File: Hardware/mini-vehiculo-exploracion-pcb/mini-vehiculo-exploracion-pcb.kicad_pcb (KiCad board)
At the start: 2 copper layers, 82 parts, among them IC3 MAX8891EXK33_V+T, J1 Cámara, J2 USB_C_Receptacle_USB2.0_16P, J4 MOTORES, J8 SERVO, Q1 SI1467DH-T1-BE3, U2 ESP32-S3-WROOM-1, U3 LM358, U4 TPS561208DDCR, Y1 830003000

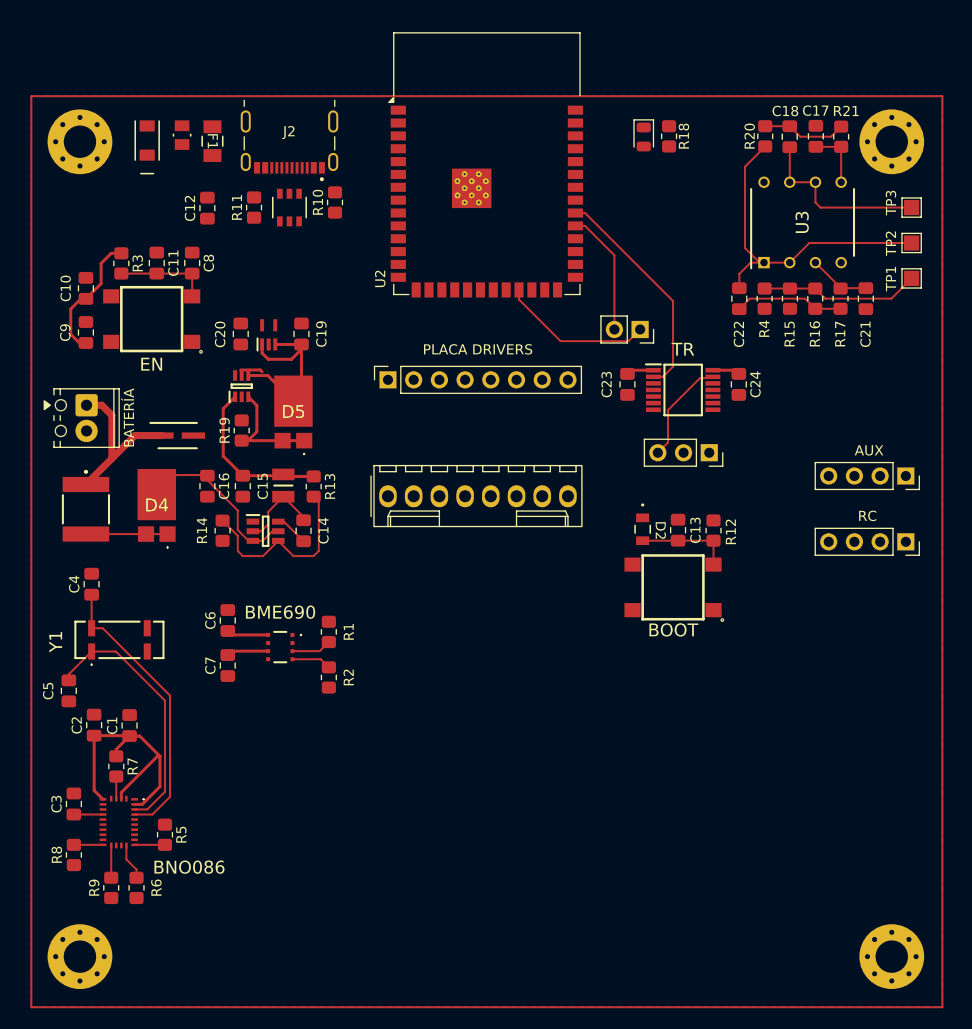
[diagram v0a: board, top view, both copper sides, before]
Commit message: update pcb3
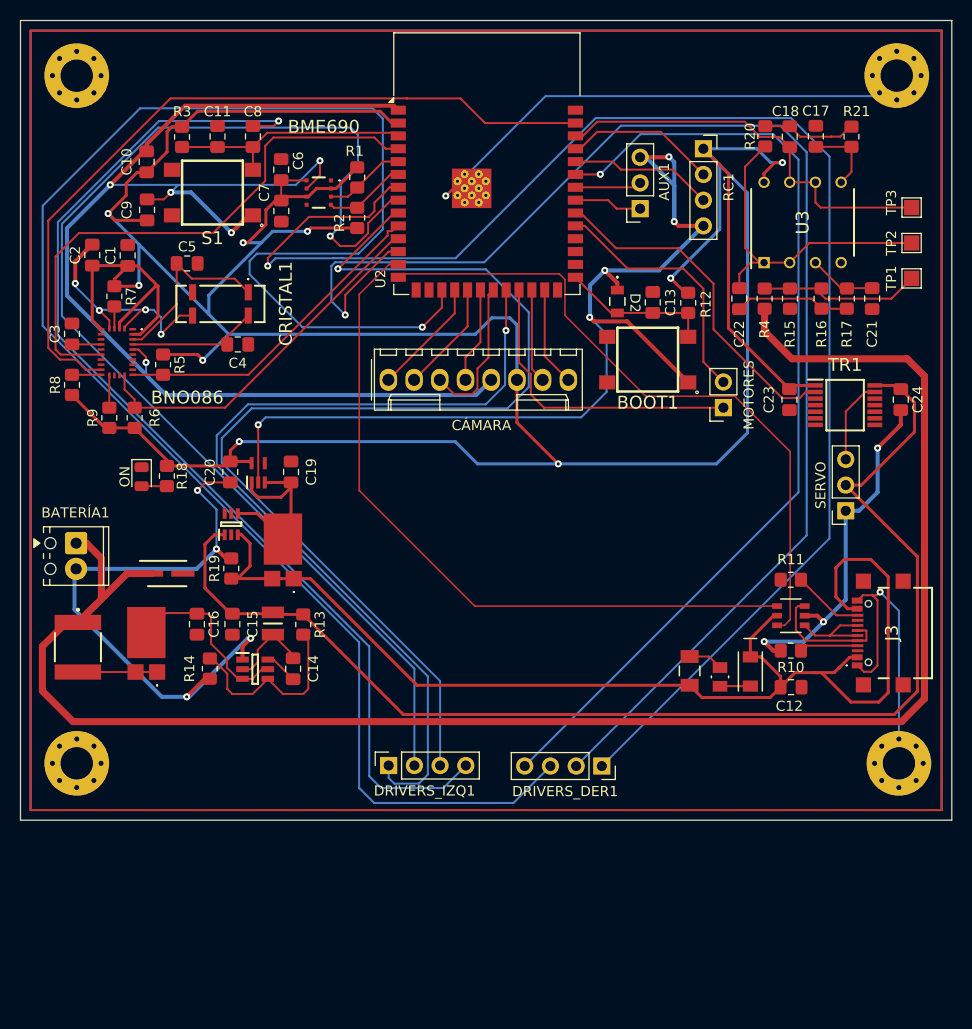
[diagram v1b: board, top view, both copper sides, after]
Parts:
- removed AUX: Aux_Conn_1x4, Connector_PinSocket_2.54mm:PinSocket_1x04_P2.54mm_Vertical
- removed J2: USB_C_Receptacle_USB2.0_16P, USB_UJ20-C-H-G-SMT-P16-TR:SAMESKY_UJ20-C-H-G-SMT-P16-TR
- removed PLACA DRIVERS: Drivers_Conn_1x8, Connector_PinSocket_2.54mm:PinSocket_1x08_P2.54mm_Vertical
- added AUX1: AUX, Connector_PinSocket_2.54mm:PinSocket_1x03_P2.54mm_Vertical, F.Cu at (146.2, 60.6)
- added DRIVERS_DER1: DRIVERS_DER, Connector_PinSocket_2.54mm:PinSocket_1x04_P2.54mm_Vertical, F.Cu at (142.5, 115.7)
- added DRIVERS_IZQ1: DRIVERS_IZQ, Connector_PinSocket_2.54mm:PinSocket_1x04_P2.54mm_Vertical, F.Cu at (121.4, 115.6)
- added J3: UJ20-C-H-G-SMT-5-P16-TR, USB_UJ20-C-H-G-SMT-P16-TR:UJ20CHGSMT5P16TR, F.Cu at (171.4, 102.5)
- J1: value Cámara -> CÁMARA
- RC1: renamed from RC; value RC_Conn_1x4 -> RC
- U2: footprint RF_Module:ESP32-S3-WROOM-1 -> ESP32-S3-WROOM-1-P3JLC:ESP32-S3-WROOM-1-P3JLC
- moved D1 79.4 mm to (157.1, 106.3), turned to -90 degrees
- moved FB1 75.4 mm to (154.1, 106.8), turned to -90 degrees
- moved C12 74.6 mm to (161.2, 107.9), turned to 0 degrees
- moved F1 70.4 mm to (151.1, 106.2), turned to 90 degrees
- moved R11 64.5 mm to (161.1, 97.2), turned to 180 degrees
- moved CR1 63.9 mm to (161.1, 100.8), turned to 180 degrees
- moved R10 63.1 mm to (161.1, 104.2), turned to 180 degrees
- moved D6 59.9 mm to (97.0, 87.1)
- moved R18 59.9 mm to (99.5, 87.0)
- moved BNO086 46.4 mm to (94.6, 74.8)
- moved C2 46.4 mm to (92.1, 65.2)
- moved R5 46.4 mm to (99.1, 76.0)
- moved R6 46.4 mm to (96.3, 81.2)
- moved R7 46.4 mm to (94.3, 69.2)
- moved R8 46.4 mm to (90.1, 78.0)
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- renumbered BATERÍA to BATERÍA1, BOOT to BOOT1, Y1 to CRISTAL1, J4 to MOTORES1, EN to S1, TR to TR1
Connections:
- C24 pad 1: V_SELEC -> V_BAT
- F1 pad 1: Net-(F1-Pad1) -> V_BUS
- J8 pad 2: V_SELEC -> V_BAT
- TR1 pad 14: V_SELEC -> V_BAT
- U2 pad 35: /PIN_AUX3 -> /ADC_BAT2
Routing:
- net GND: track 0.00 -> 544.9 mm, vias 0 -> 24
- net +3.3V: track 54.7 -> 350.0 mm, vias 0 -> 9
- net /M1_DISABLE: track 0.00 -> 179.9 mm, vias 0 -> 1
- net /M1_IN1: track 0.00 -> 149.7 mm, vias 0 -> 1
- net ENT_BAT: track 16.7 -> 166.3 mm
- net /M1_IN2: track 0.00 -> 138.3 mm, vias 0 -> 1
- net /M2_IN2: track 0.00 -> 122.1 mm, vias 0 -> 1
- net /M2_DISABLE: track 0.00 -> 110.0 mm, vias 0 -> 1
- net V_BAT: track 16.2 -> 123.0 mm
- net V_BUS: track 11.9 -> 116.8 mm
- net /ADC_BAT2: track 0.00 -> 95.8 mm, vias 0 -> 1
- net /M2_IN1: track 0.00 -> 87.8 mm, vias 0 -> 1
- net /BNO_INT: track 0.00 -> 76.8 mm
- net USB_D-: track 0.00 -> 70.5 mm
- net USB_D+: track 0.00 -> 66.3 mm
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- added copper zone on F.Cu, net GND
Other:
- board outline added: 92 x 79 mm
